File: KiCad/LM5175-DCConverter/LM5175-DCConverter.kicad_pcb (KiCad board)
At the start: 4 copper layers, 103 parts, among them J1 Conn_01x02, J2 Conn_01x02, J3 REX128128AYAP3N00000, J4 SWD, Q1 CSD18534, Q2 CSD18511, Q3 CSD18534, Q4 CSD18511, Q5 IRLML2502, SW1 SW_DIP_x01, SW2 SW_DIP_x01, SW3 SW_DIP_x01, U1 LM5175PWP, U2 INA233, U3 STM32L051K8Tx, U4 MCP9800, U5 L7815, U6 L78L33_SOT89, U7 MCP9800, U8 INA233

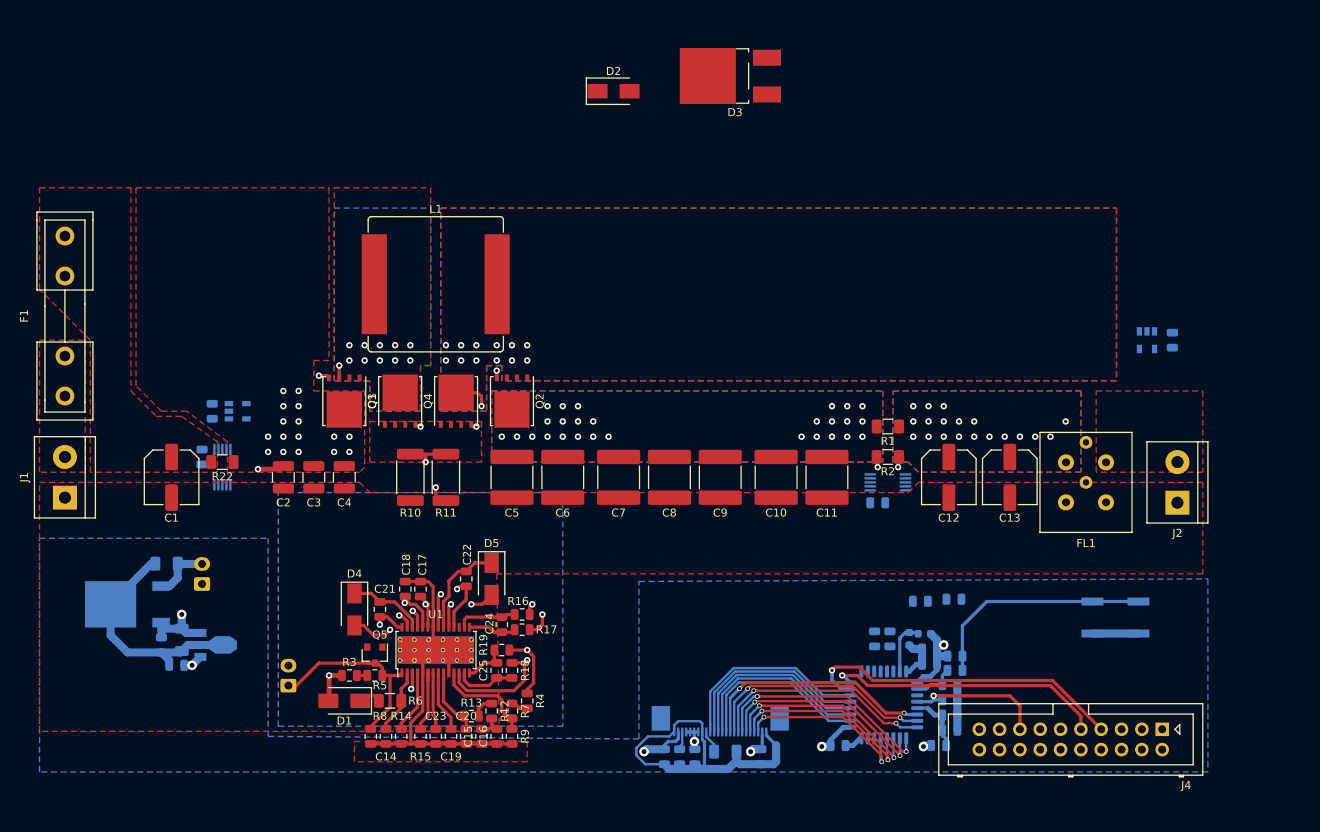
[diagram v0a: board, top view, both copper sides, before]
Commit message: Most of the PCB done
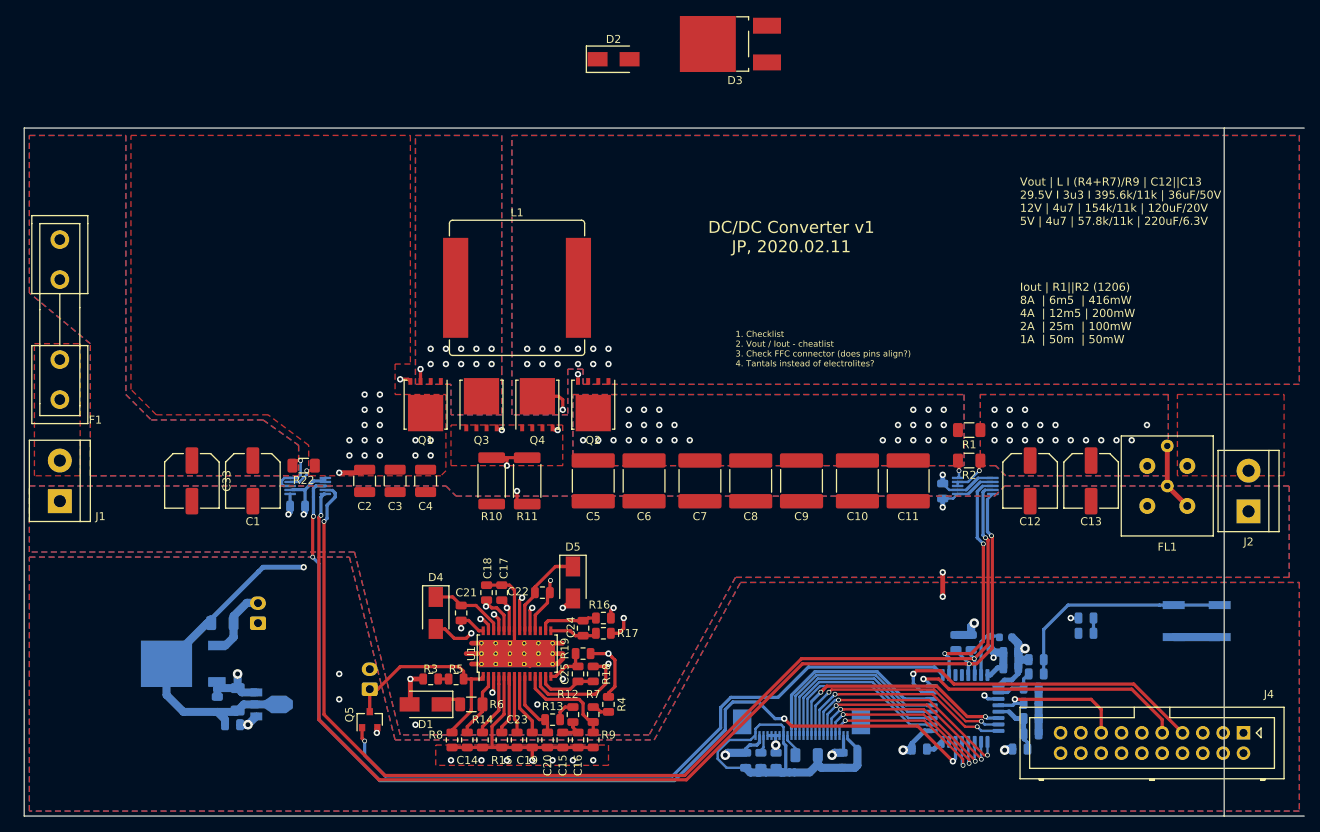
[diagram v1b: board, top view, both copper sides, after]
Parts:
- removed C38: 100n, Capacitor_SMD:C_0805_2012Metric
- removed REF**: REX128128AYAP3N00000, JPDisplays:REX128128AYAP3N00000
- removed U4, U7: MCP9800, Package_TO_SOT_SMD:SOT-23-5
- C33: value 100n -> 100u/35V; footprint Capacitor_SMD:C_0805_2012Metric -> Capacitor_SMD:C_Elec_6.3x7.7; moved to F.Cu
- moved C33 123.8 mm to (101.0, 74.1)
- moved D6 20.8 mm to (212.7, 91.2)
- moved R26 17.0 mm to (212.7, 93.2), turned to 180 degrees
- moved C41 13.4 mm to (114.2, 77.3), turned to 0 degrees
- moved U2 10.9 mm to (198.9, 74.7)
- moved U8 10.9 mm to (115.4, 74.7), turned to 180 degrees
- moved C34 10.2 mm to (104.8, 91.9)
- moved C35 10.2 mm to (104.1, 102.0)
- moved C36 10.2 mm to (106.7, 101.4)
- moved U5 10.2 mm to (99.9, 97.0)
- moved U6 10.2 mm to (110.5, 102.0)
- moved C37 10.2 mm to (106.0, 104.6)
- moved C13 10.2 mm to (213.4, 74.1)
- moved C24 10.2 mm to (149.9, 92.5)
- moved R13 10.2 mm to (146.1, 104.0)
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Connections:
- C14 pad 2: CSG -> GNDA
- C15 pad 1: CSG -> GNDA
- C16 pad 1: CSG -> GNDA
- C19 pad 1: CSG -> GNDA
- C20 pad 1: CSG -> GNDA
- C23 pad 1: CSG -> GNDA
- C26 pad 2: CSG -> GNDA
- C27 pad 2: CSG -> GNDA
- C28 pad 2: CSG -> GNDA
- C29 pad 2: CSG -> GNDA
- C30 pad 2: CSG -> GNDA
- C31 pad 2: CSG -> GNDA
- C32 pad 2: CSG -> GNDA
- C33 pad 1: +3V3 -> Vin+
- C34 pad 2: CSG -> GNDA
- C35 pad 2: CSG -> GNDA
- C36 pad 2: CSG -> GNDA
- C37 pad 2: CSG -> GNDA
- C39 pad 1: CSG -> GNDA
- C40 pad 2: CSG -> GNDA
- C41 pad 2: CSG -> GNDA
- C42 pad 2: CSG -> GNDA
- C44 pad 2: CSG -> GNDA
- C45 pad 2: CSG -> GNDA
- J3 pad 1: CSG -> GNDA
- J3 pad 24: CSG -> GNDA
- J3 pad 8: CSG -> GNDA
- J4 pad 10: CSG -> GNDA
- J4 pad 12: CSG -> GNDA
- J4 pad 14: CSG -> GNDA
- J4 pad 18: CSG -> GNDA
- J4 pad 20: CSG -> GNDA
- J4 pad 3: CSG -> GNDA
- J4 pad 4: CSG -> GNDA
- J4 pad 6: CSG -> GNDA
- J4 pad 8: CSG -> GNDA
- Q5 pad 2: CSG -> GNDA
- R14 pad 2: CSG -> GNDA
- R15 pad 2: CSG -> GNDA
- R21 pad 2: CSG -> GNDA
- R23 pad 2: CSG -> GNDA
- R26 pad 2: CSG -> GNDA
- R8 pad 2: CSG -> GNDA
- R9 pad 2: CSG -> GNDA
- SW2 pad 2: CSG -> GNDA
- SW3 pad 2: CSG -> GNDA
- U1 pad 10: CSG -> GNDA
- U1 pad 5: CSG -> GNDA
- U2 pad 1: CSG -> GNDA
- U2 pad 7: CSG -> GNDA
- U3 pad 16: CSG -> GNDA
- U3 pad 25: Net-(U3-Pad25) -> ShutOff
- U3 pad 28: ShutOff -> Net-(U3-Pad28)
- U3 pad 32: CSG -> GNDA
- U5 pad 2: CSG -> GNDA
- U6 pad 2: CSG -> GNDA
- U8 pad 1: CSG -> GNDA
- U8 pad 2: CSG -> GNDA
- U8 pad 7: CSG -> GNDA
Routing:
- net GNDA: track 0.00 -> 182.6 mm, vias 0 -> 14
- net SDA: track 0.00 -> 146.6 mm, vias 0 -> 3
- net SCL: track 0.00 -> 146.4 mm, vias 0 -> 3
- net InaInAlert: track 0.00 -> 124.5 mm, vias 0 -> 4
- net CSG: track 163.2 -> 67.6 mm, vias 2 -> 5
- net ShutOff: track 0.00 -> 84.4 mm, vias 0 -> 1
- net +3V3: track 172.1 -> 244.2 mm, vias 5 -> 10
- net InaOutAlert: track 0.00 -> 29.7 mm, vias 0 -> 2
- net LED: track 0.00 -> 17.7 mm, vias 0 -> 2
- net Vin-: track 57.6 -> 66.2 mm, vias 19 -> 20
- net Vin+: track 0.00 -> 7.29 mm, vias 0 -> 1
- net +15V: track 100.2 -> 106.6 mm
- net Isense-: track 104.3 -> 108.1 mm
- net EN: track 24.1 -> 26.9 mm
- net Net-(D6-Pad1): track 0.00 -> 1.91 mm
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- added copper zone on F.Cu, net +3V3
- added copper zone on B.Cu, net GNDA
- added copper zone on F.Cu, net GNDA
- added copper zone on B.Cu, net Vin+
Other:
- board outline added: 160 x 86 mm
- net class Big added: clearance 0.1778, trace_width 0.6096, via_dia 0.8, via_drill 0.4
- net class Default: clearance 0.2 -> 0.1778; via_dia 0.8 -> 0.6
- net class Power: clearance 0.2 -> 0.1778
- rule trace_clearance: 0.2 -> 0.1778
- board text added: "1. Checklist 2. Vout / Iout - cheatlist 3. Check FFC connector (does pins align?) 4. Tantals instead of electrolites?"
- board text added: "DC/DC Converter v1 JP, 2020.02.11"
- board text added: "Iout | R1||R2 (1206) 8A | 6m5 | 416mW 4A | 12m5 | 200mW 2A | 25m | 100mW 1A | 50m | 50mW"
- board text added: "Vout | L I (R4+R7)/R9 | C12||C13 29.5V I 3u3 I 395.6k/11k | 36uF/50V 12V | 4u7 | 154k/11k | 120uF/20V 5V | 4u7 | 57.8k/11k | 220uF/6.3V"
